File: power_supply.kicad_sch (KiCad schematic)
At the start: 21 parts, among them IC2 CH224K, IC8 MP1584EN, J2 USB4940-00-A

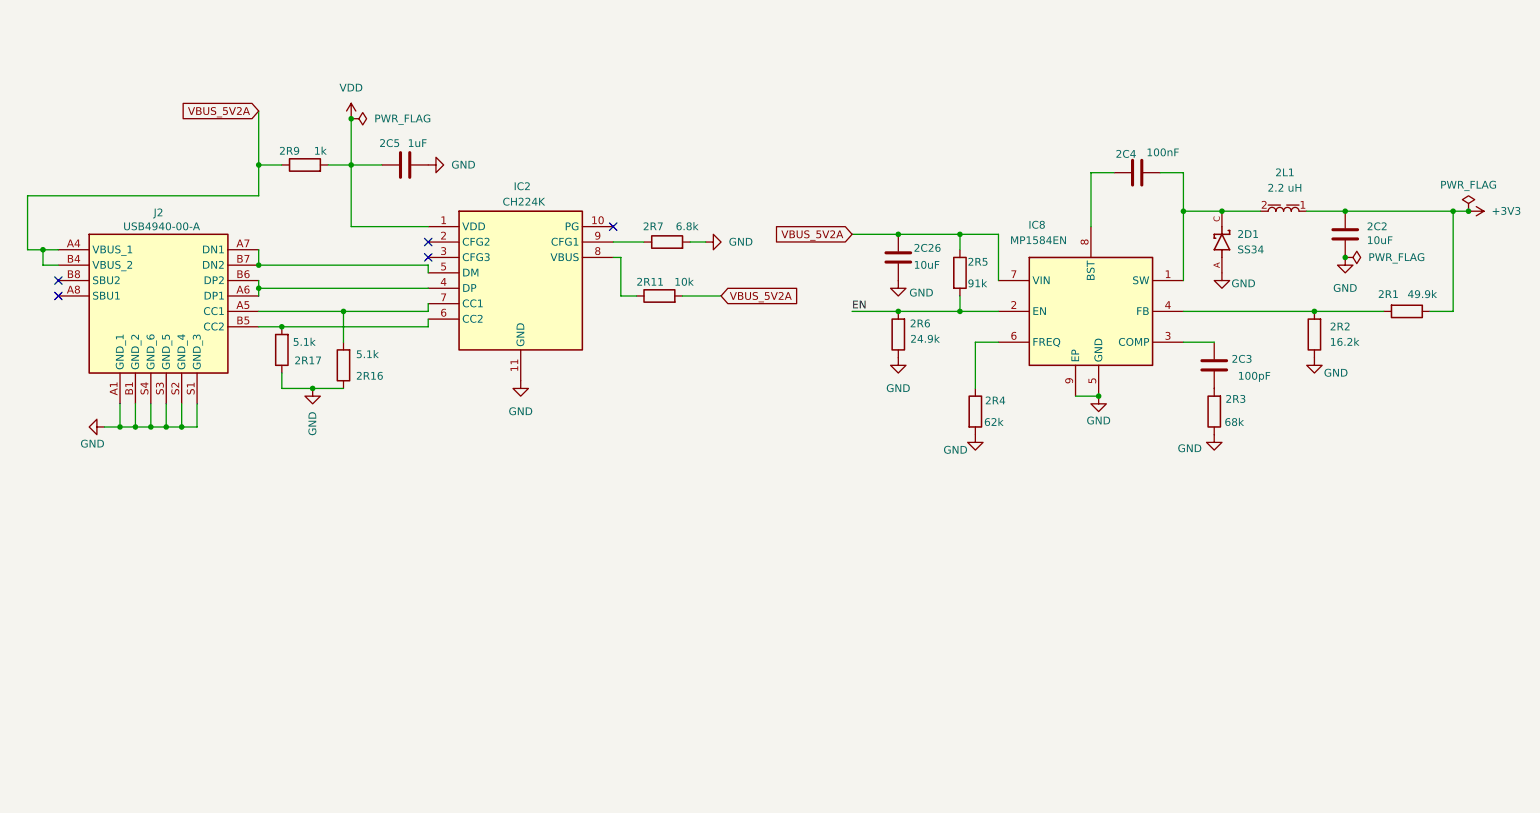
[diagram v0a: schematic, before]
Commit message: finalize power and esp schemas
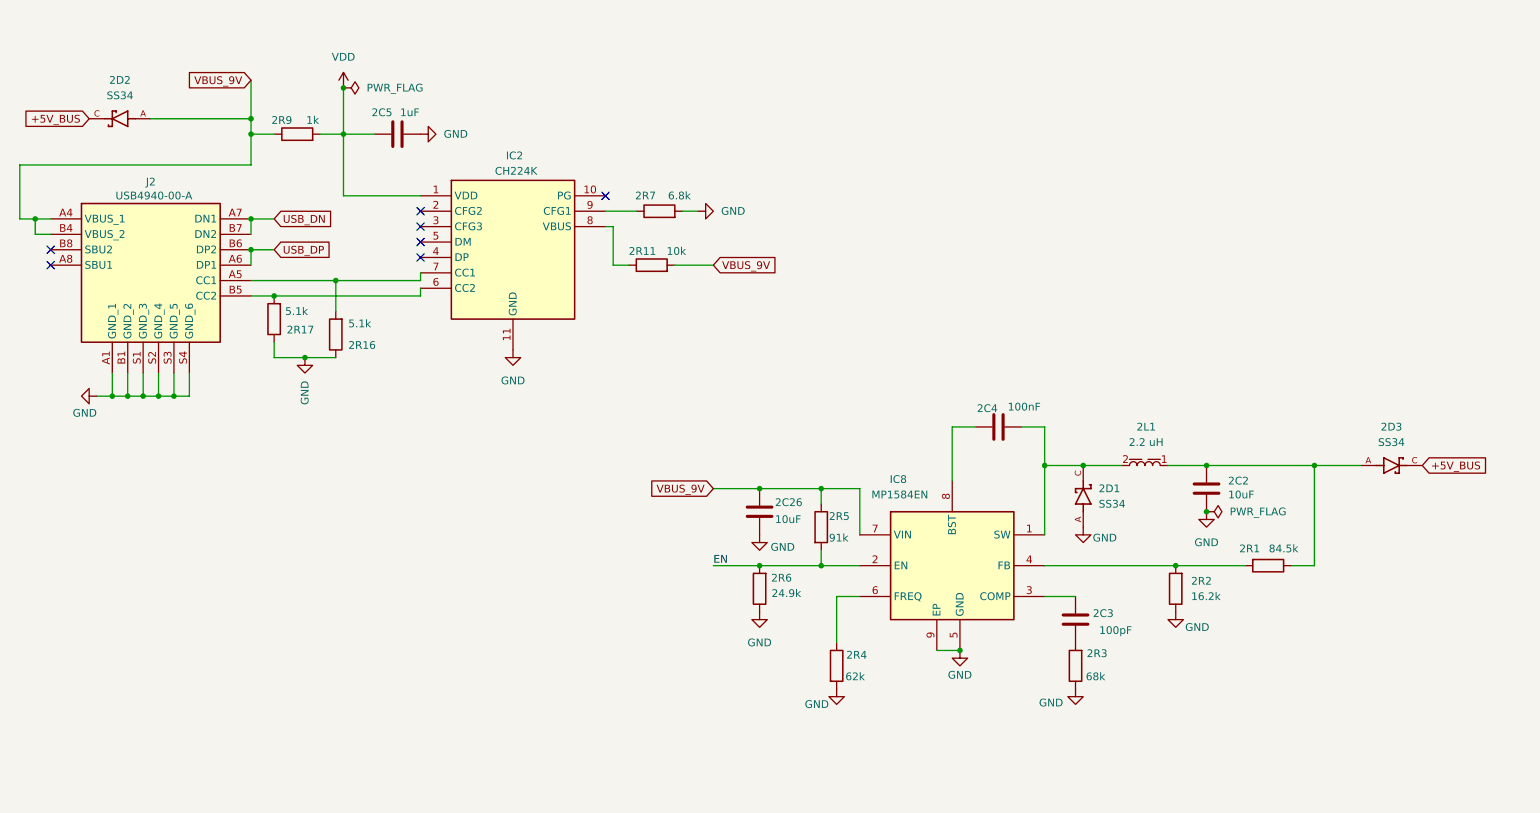
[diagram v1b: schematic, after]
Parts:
- added 2D2, 2D3: SS34, ipradio:DIOM7959X265N, symbol ipradio:SS34
- 2R1: value 49.9k -> 84.5k
- J2: symbol esp32_selfmade_Esp_32_module:USB4940-00-A -> ipradio:USB4940-00-A
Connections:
- net USB_DP: now reaches J2.A6 (DP1), J2.B6 (DP2)
- net USB_DP: no longer IC2.4 (DP)
- net USB_DN: now reaches J2.A7 (DN1), J2.B7 (DN2)
- net USB_DN: no longer IC2.5 (DM)
- net +3V3: no longer names the net of 2C2.1, 2L1.1, 2R1.1
- net +3V3: now also 2D3.A
- net VBUS_5V2A renamed VBUS_9V
- net VBUS_9V: now also 2D2.A
- new net +5V_BUS: 2D2.C, 2D3.C
- no-connect marks 5 -> 7
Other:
- moved on the sheet: 2C2, 2C26, 2C3, 2C4, 2C5, 2D1, 2L1, 2R1, 2R11, 2R16, 2R17, 2R2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

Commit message: finalized schema
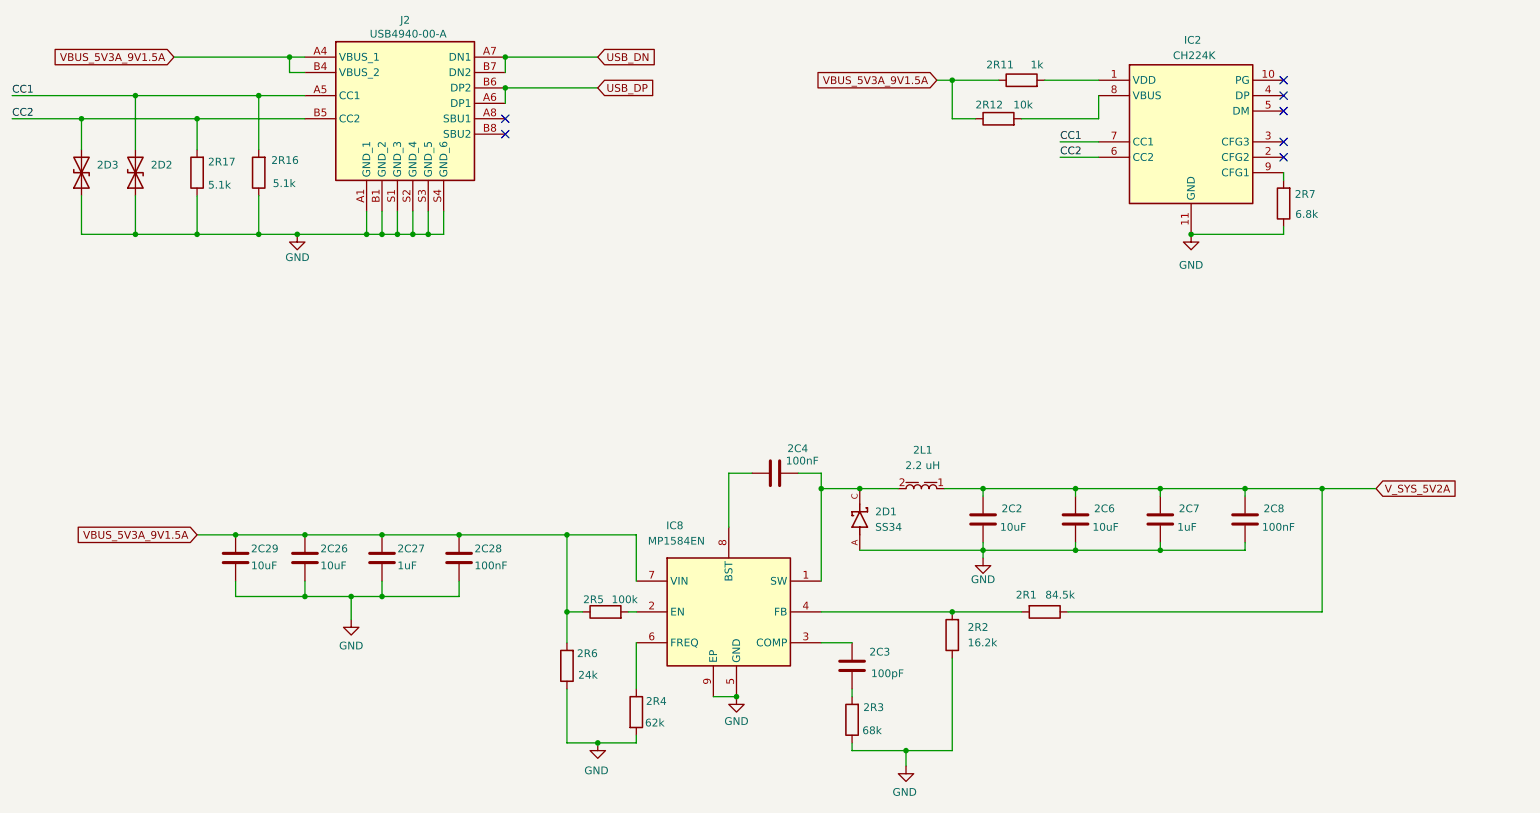
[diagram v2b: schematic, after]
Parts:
- removed 2C5: 1uF, Capacitor_SMD:C_0402_1005Metric, symbol Device:C
- removed 2D2, 2D3: SS34, ipradio:DIOM7959X265N, symbol ipradio:SS34
- removed 2R9: 1k, Resistor_SMD:R_0402_1005Metric, symbol Device:R
- added 2C27: 1uF, Capacitor_SMD:C_1206_3216Metric, symbol Device:C
- added 2C28: 100nF, Capacitor_SMD:C_1206_3216Metric, symbol Device:C
- added 2C29: 10uF, Capacitor_SMD:C_1206_3216Metric, symbol Device:C
- added 2C6: 10uF, Capacitor_SMD:C_0805_2012Metric, symbol Device:C
- added 2C7: 1uF, Capacitor_SMD:C_0805_2012Metric, symbol Device:C
- added 2C8: 100nF, Capacitor_SMD:C_0805_2012Metric, symbol Device:C
- added 2D2, 2D3: D_TVS, Diode_SMD:D_SOD-123, symbol Device:D_TVS
- added 2R12: 10k, Resistor_SMD:R_0402_1005Metric, symbol Device:R
- 2R11: value 10k -> 1k
- 2R5: value 91k -> 100k
- 2R6: value 24.9k -> 24k
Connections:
- net GND: now also 2R7.1, 2C27.2, 2C28.2, 2C29.2, 2C6.2, 2C7.2, 2C8.2, 2D2.1 (A1), 2D3.1 (A1); no longer 2R7.2
- net CC1: now reaches 2R16.2, IC2.7 (CC1), J2.A5 (CC1)
- net CC1: now also 2D2.2 (A2)
- net CC2: now reaches 2R17.2, IC2.6 (CC2), J2.B5 (CC2)
- net CC2: now also 2D3.2 (A2)
- net V_SYS_5V2A: now reaches 2C2.1, 2L1.1, 2R1.1
- net V_SYS_5V2A: now also 2C6.1, 2C7.1, 2C8.1
- net at IC2.8 (VBUS): now also 2R12.2; no longer 2R11.1
- net at IC2.9 (CFG1): now also 2R7.2; no longer 2R7.1
- net EN: no longer names the net of 2R5.2, IC8.2 (EN)
- net EN: no longer 2R6.2
- net VBUS_9V renamed VBUS_5V3A_9V1.5A
- net VBUS_5V3A_9V1.5A: now also 2R11.1, 2R6.2, 2C27.1, 2C28.1, 2C29.1, 2R12.1; no longer 2R11.2
- net VDD: no longer names the net of IC2.1 (VDD)
- net VDD: now also 2R11.2
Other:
- moved on the sheet: 2C2, 2C26, 2C3, 2C4, 2D1, 2L1, 2R1, 2R16, 2R17, 2R2, 2R3, 2R4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
